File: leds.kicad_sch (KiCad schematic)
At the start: 29 parts, among them J18 LED-Ring, J19 LED-Ring, J20 LED-Ring, J21 LED-Ring, J22 LED-Ring, J23 LED-Ring, J4 RGB_LED_EXT, U3 74AHCT1G32SE-7

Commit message: Replace reverse power diode with MOSFET
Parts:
- U3: Check_prices https://www.snapeda.com/parts/74AHCT1G32SE-7/Diodes+Inc./vi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 -> (none)
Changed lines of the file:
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@@
-      (effects (font (size 1.27 1.27)) (justify bottom) hide)
-    )
-    (property "Check_prices" "https://www.snapeda.com/parts/74AHCT1G32SE-7/Diodes+Inc./view-part/?ref=eda" (at 100.33 50.8 0)
       (effects (font (size 1.27 1.27)) (justify bottom) hide)
     )

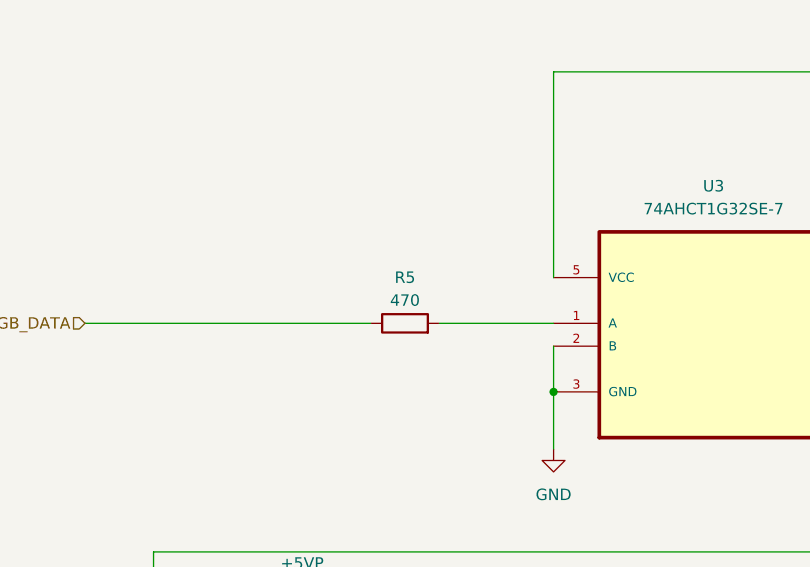
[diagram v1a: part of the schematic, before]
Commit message: Replace capacitors for PSU with SMD components
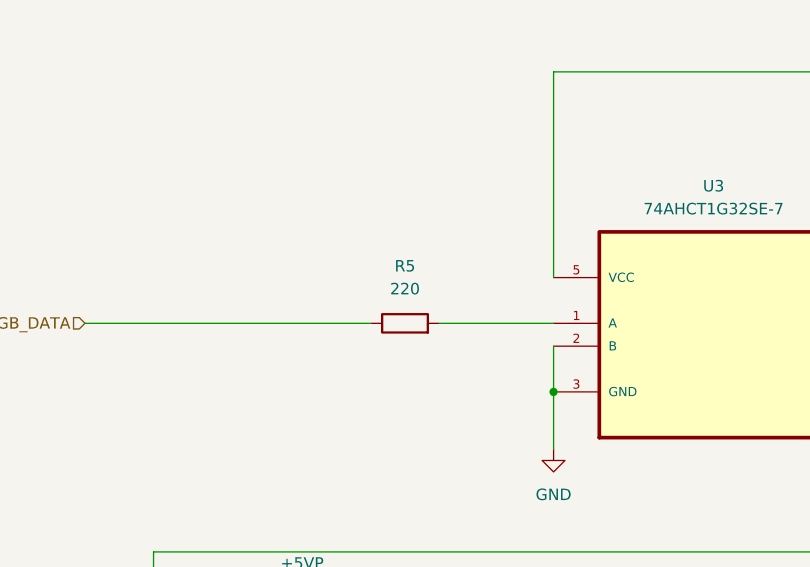
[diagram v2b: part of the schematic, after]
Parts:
- R5: value 470 -> 220
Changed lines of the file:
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@@
   (symbol (lib_id "Device:R") (at 66.04 53.34 90) (unit 1)
     (in_bom yes) (on_board yes) (dnp no) (fields_autoplaced)
-    (property "Reference" "R5" (at 66.04 48.26 90)
+    (property "Reference" "R5" (at 66.04 46.99 90)
       (effects (font (size 1.27 1.27)))
     )
-    (property "Value" "470" (at 66.04 50.8 90)
+    (property "Value" "220" (at 66.04 49.53 90)
       (effects (font (size 1.27 1.27)))
     )
@@
         )
         (path "/df521c2a-9827-4355-b809-366f4b88d5d7/539b926e-3ef4-477a-b921-49e2b2b26dfc"
-          (reference "R5") (unit 1)
+          (reference "R4") (unit 1)
         )
       )

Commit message: Fix ERC errors
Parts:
- U3: footprint Package_TO_SOT_SMD:SOT-353_SC-70-5 -> Pedalboard Library:SOT65P210X110-5N
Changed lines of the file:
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@@
         )
         (path "/df521c2a-9827-4355-b809-366f4b88d5d7/539b926e-3ef4-477a-b921-49e2b2b26dfc"
-          (reference "R4") (unit 1)
+          (reference "R5") (unit 1)
         )
       )
@@
       (effects (font (size 1.27 1.27)))
     )
-    (property "Footprint" "Package_TO_SOT_SMD:SOT-353_SC-70-5" (at 100.33 50.8 0)
+    (property "Footprint" "Pedalboard Library:SOT65P210X110-5N" (at 100.33 50.8 0)
       (effects (font (size 1.27 1.27)) (justify bottom) hide)
     )

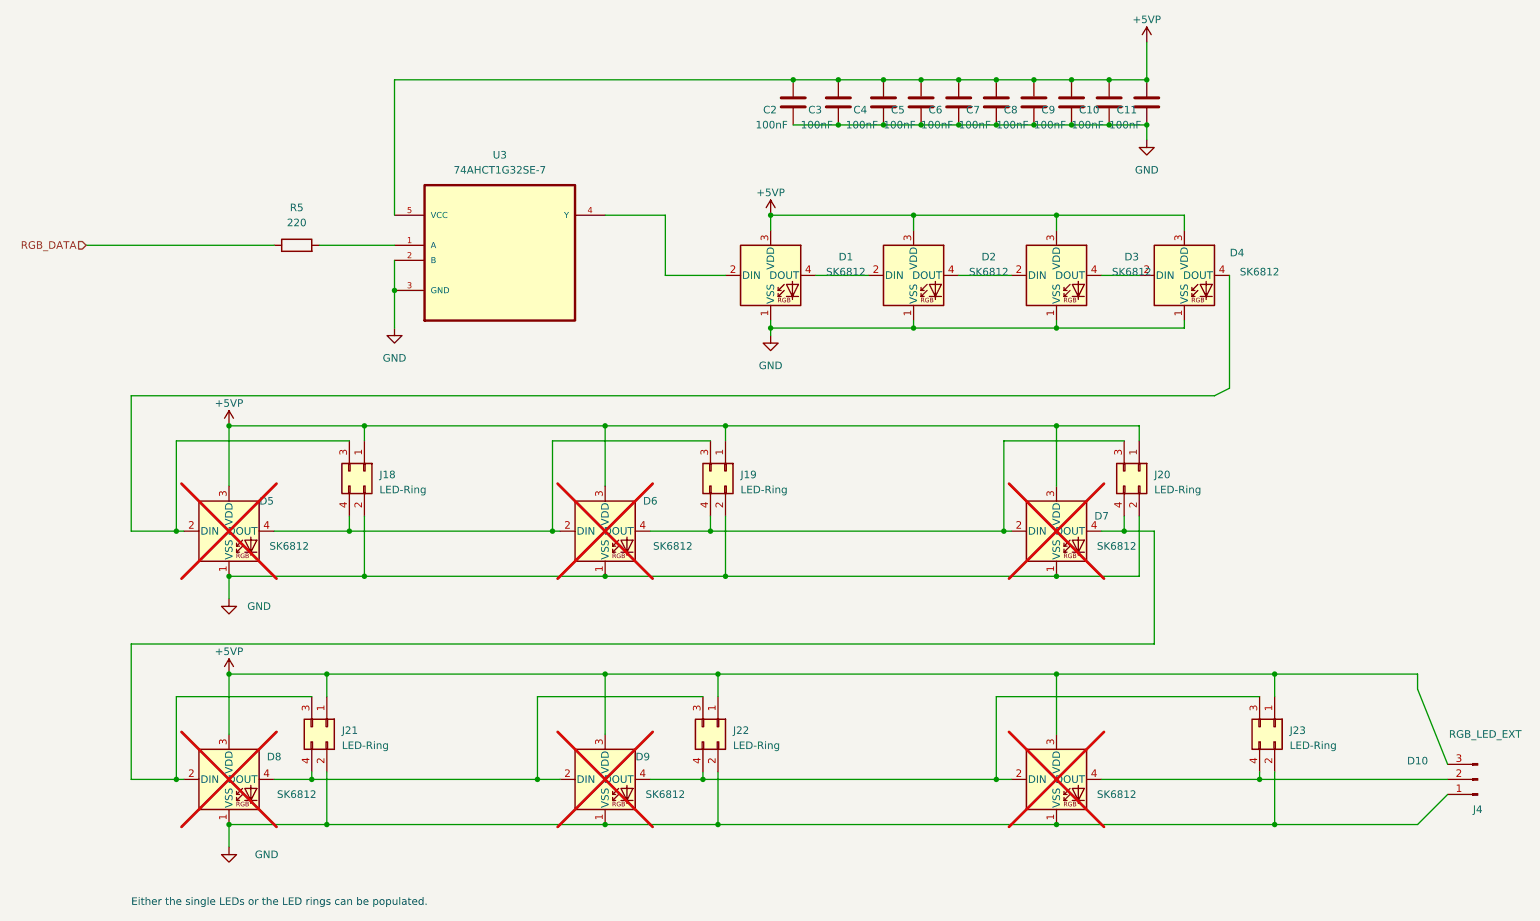
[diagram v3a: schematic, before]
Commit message: Started to cleanup routing
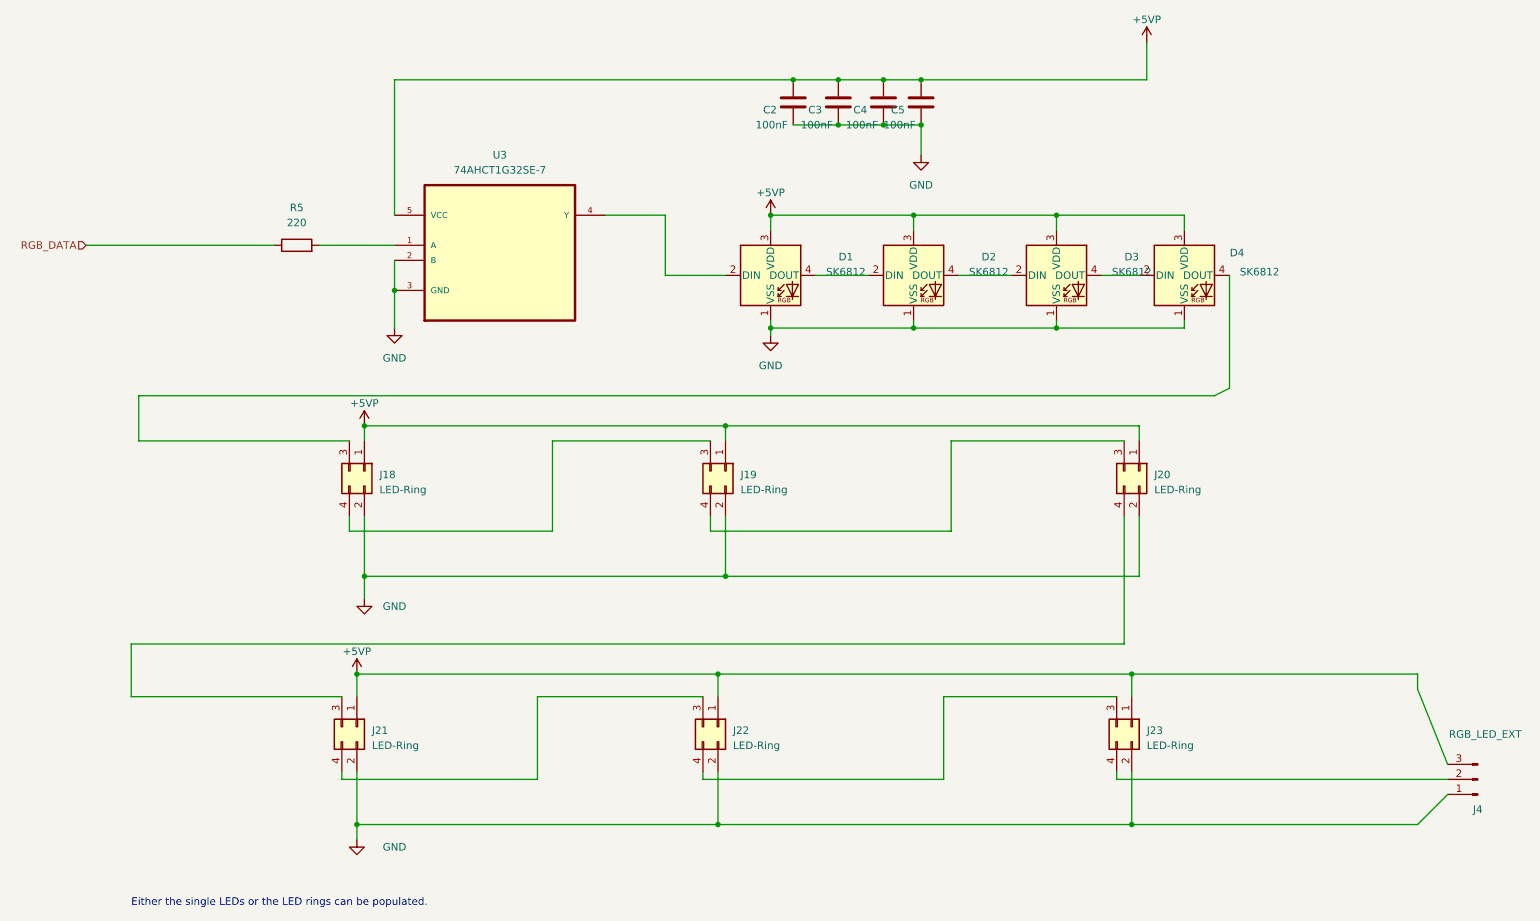
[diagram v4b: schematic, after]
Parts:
- removed C10, C11, C6, C7, C8, C9: 100nF, Capacitor_SMD:C_0805_2012Metric, symbol Device:C
- removed D10, D5, D6, D7, D8, D9: SK6812, LED_SMD:LED_SK6812_PLCC4_5.0x5.0mm_P3.2mm, symbol LED:SK6812
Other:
- moved on the sheet: J21, J23

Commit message: Resize PCB
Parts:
- J4: footprint Connector_PinHeader_2.54mm:PinHeader_1x03_P2.54mm_Horizontal -> Connector_JST:JST_XH_B3B-XH-A_1x03_P2.50mm_Vertical
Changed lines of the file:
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@@
       (effects (font (size 1.27 1.27)))
     )
-    (property "Footprint" "Connector_PinHeader_2.54mm:PinHeader_1x03_P2.54mm_Horizontal" (at 265.43 143.51 0)
+    (property "Footprint" "Connector_JST:JST_XH_B3B-XH-A_1x03_P2.50mm_Vertical" (at 265.43 143.51 0)
       (effects (font (size 1.27 1.27)) hide)
     )

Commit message: Driver for LED
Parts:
- U3: footprint Pedalboard Library:SOT65P210X110-5N -> SOT-353_SC-70-5
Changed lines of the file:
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@@
       (effects (font (size 1.27 1.27)))
     )
-    (property "Footprint" "Pedalboard Library:SOT65P210X110-5N" (at 100.33 50.8 0)
+    (property "Footprint" "SOT-353_SC-70-5" (at 100.33 50.8 0)
       (effects (font (size 1.27 1.27)) (justify bottom) hide)
     )
